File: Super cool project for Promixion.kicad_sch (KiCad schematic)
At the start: 8 parts, among them U1 OPA170AIDBVR

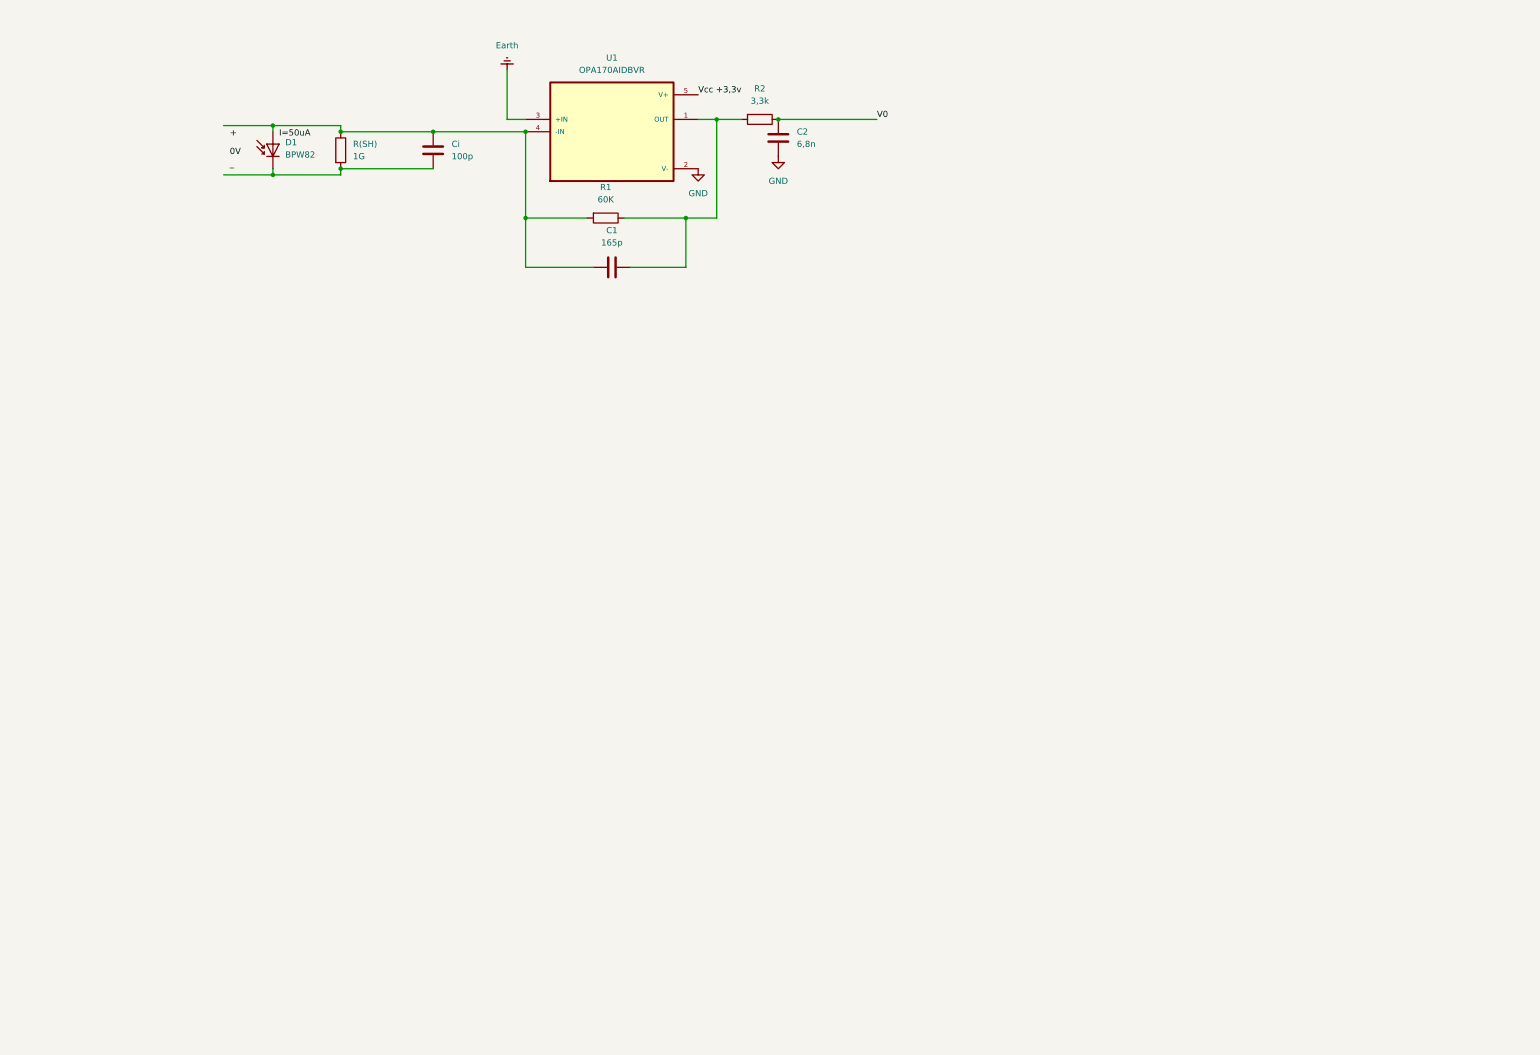
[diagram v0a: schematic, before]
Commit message: Uppdaterat KiCad-projekt med senaste ändringar
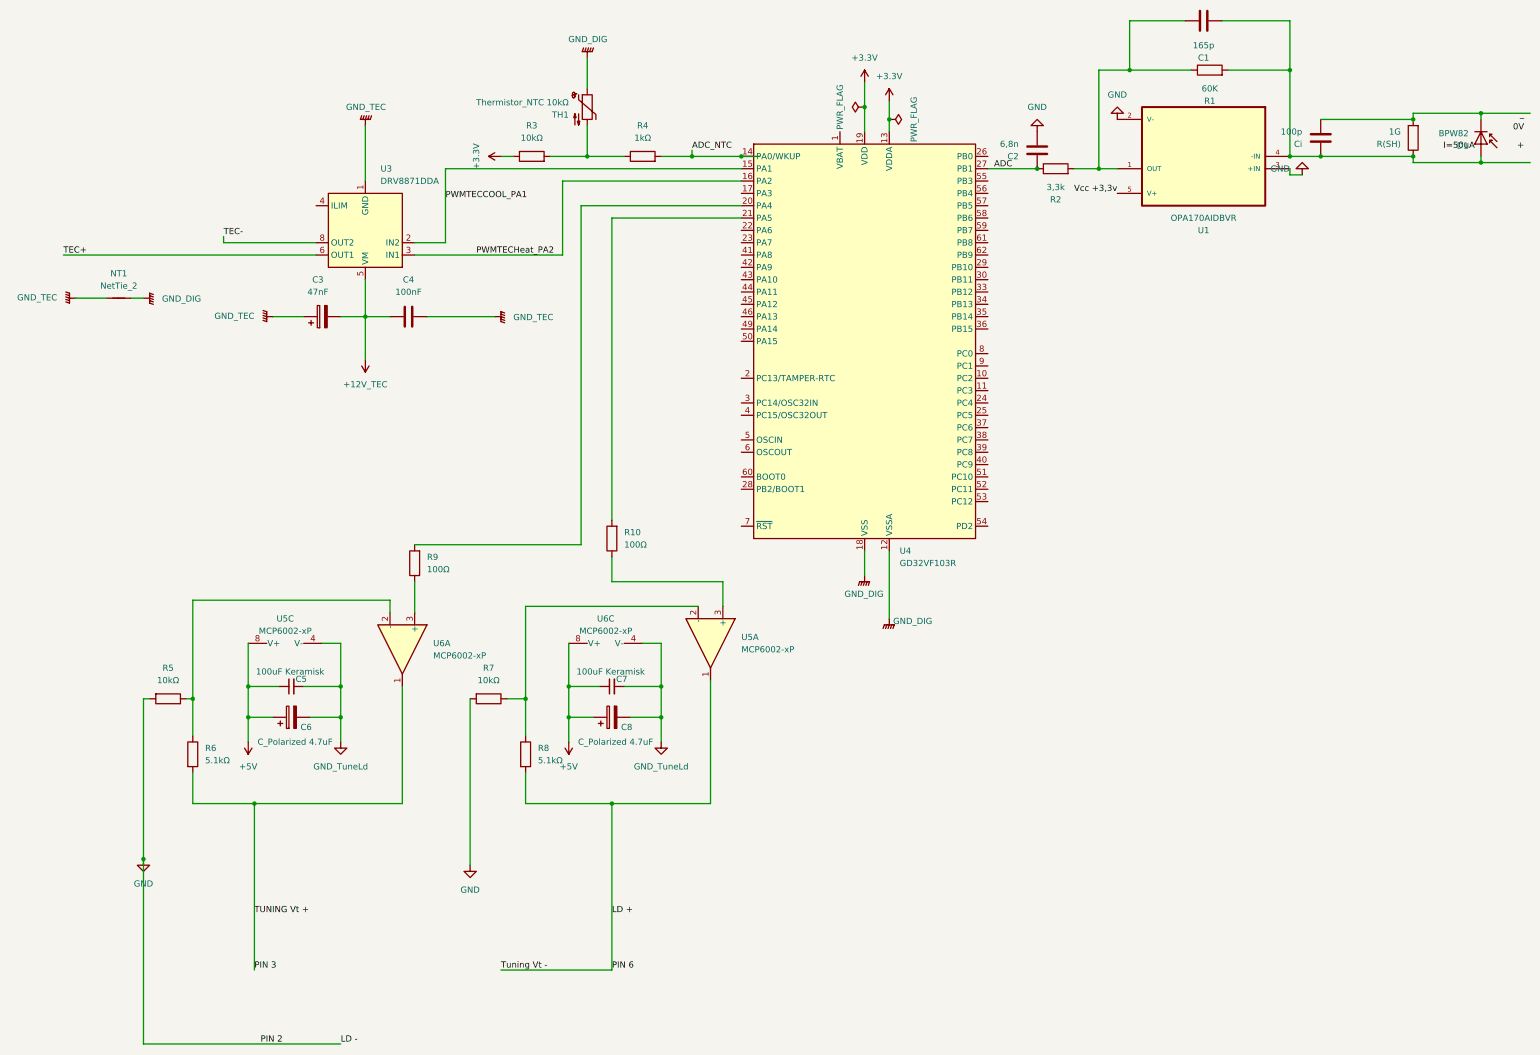
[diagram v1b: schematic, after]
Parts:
- added C3: 47nF, symbol Device:C_Polarized
- added C4: 100nF, symbol Device:C
- added C5, C7: 100uF Keramisk, symbol Device:C_Small
- added C6, C8: C_Polarized 4.7uF, symbol Device:C_Polarized
- added NT1: NetTie_2, symbol Device:NetTie_2
- added R10, R9: 100Ω, symbol Device:R
- added R3, R5, R7: 10kΩ, symbol Device:R
- added R4: 1kΩ, symbol Device:R
- added R6, R8: 5.1kΩ, symbol Device:R
- added TH1: Thermistor_NTC 10kΩ, symbol Device:Thermistor_NTC
- added U3: DRV8871DDA, Package_SO:Texas_HTSOP-8-1EP_3.9x4.9mm_P1.27mm_EP2.95x4.9mm_Mask2.4x3.1mm_ThermalVias, symbol Driver_Motor:DRV8871DDA
- added U4: GD32VF103R, Package_QFP:LQFP-64_10x10mm_P0.5mm, symbol MCU_GigaDevice:GD32VF103R
- added U5, U6: MCP6002-xP, symbol Amplifier_Operational:MCP6002-xP
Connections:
- net Earth is gone; now on net GND: U1.3 (+IN)
- net GND: now also R5.2, R7.2
- net V0 renamed ADC
- net ADC: now also U4.27 (PB1)
- new net: R5.1, R6.1, U6.2 (-)
- new net: R9.1, U6.3 (+)
- new net: R9.2, U4.20 (PA4)
- new net: R10.2, U4.21 (PA5)
- new net: R3.2, R4.1, TH1.2
- new net: R7.1, R8.1, U5.2 (-)
- new net: R10.1, U5.3 (+)
- new net +12V_TEC: C3.2, C4.1, U3.5 (VM)
- new net +3.3V: R3.1, U4.13 (VDDA), U4.19 (VDD), U4.32 (VDD), U4.48 (VDD), U4.64 (VDD)
- new net +5V: C5.1, C6.1, C7.1, C8.1, U5.8 (V+), U6.8 (V+)
- new net ADC_NTC: R4.2, U4.14 (PA0/WKUP)
- new net GND_DIG: NT1.2, TH1.1, U4.12 (VSSA), U4.18 (VSS), U4.31 (VSS), U4.47 (VSS), U4.63 (VSS)
- new net GND_TEC: C3.1, C4.2, NT1.1, U3.1 (GND), U3.7 (GND), U3.9 (GND)
- new net GND_TuneLd: C5.2, C6.2, C7.2, C8.2, U5.4 (V-), U6.4 (V-)
- new net LD +: R8.2, U5.1
- new net PIN 3: R6.2, U6.1
- new net PWMTECCOOL_PA1: U3.2 (IN2), U4.15 (PA1)
- new net PWMTECHeat_PA2: U3.3 (IN1), U4.16 (PA2)
- new net TEC+: U3.6 (OUT1)
- new net TEC-: U3.8 (OUT2)
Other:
- moved on the sheet: C1, C2, Ci, D1, R(SH), R1, R2, U1
